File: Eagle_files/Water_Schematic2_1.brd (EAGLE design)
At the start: 25.7 x 32.6 mm, 8 parts

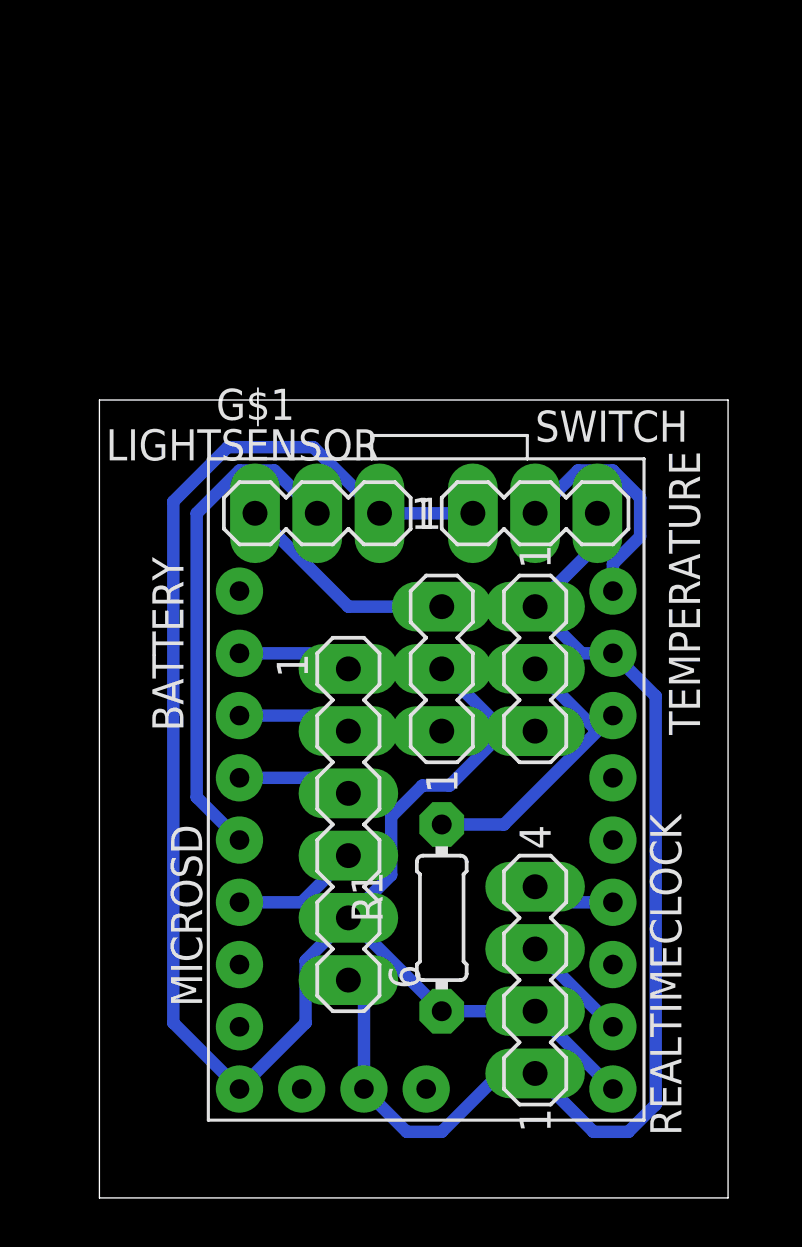
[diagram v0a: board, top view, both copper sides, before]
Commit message: Eagle files updated
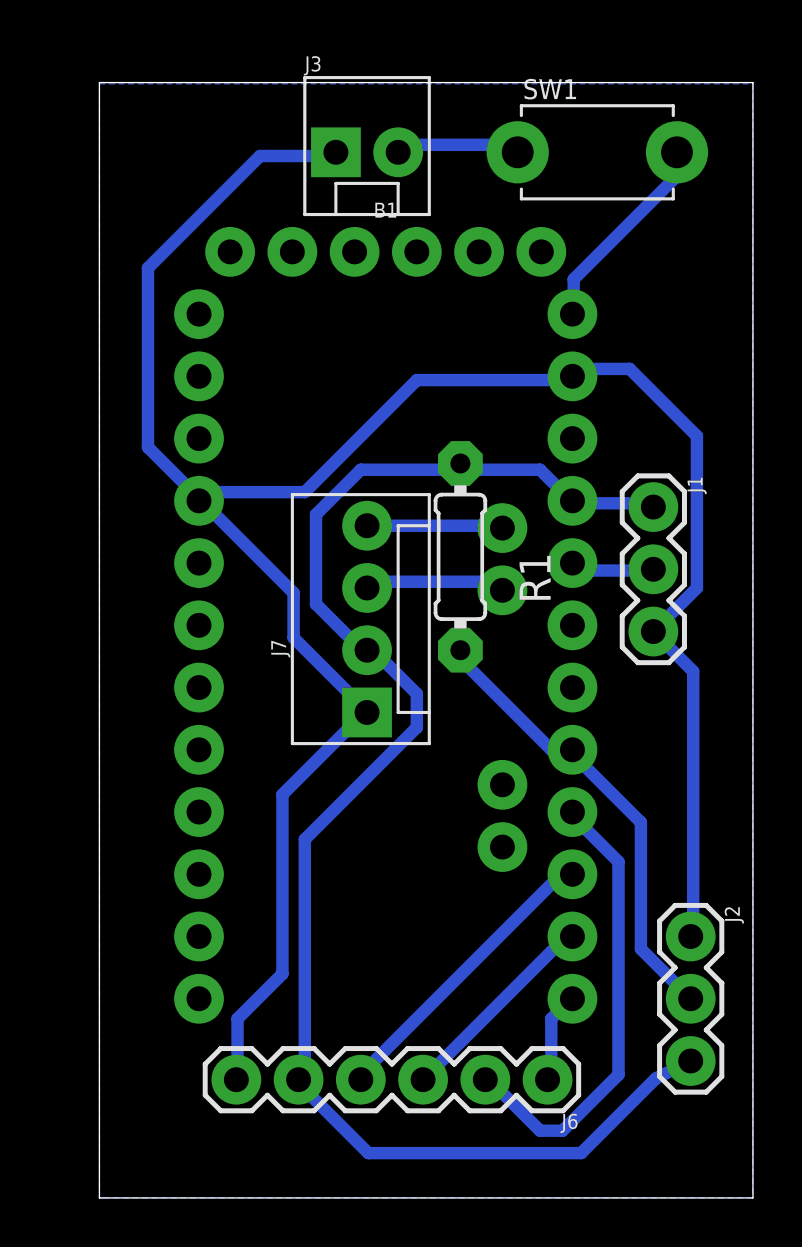
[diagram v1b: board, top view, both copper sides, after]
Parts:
- removed BATTERY, LIGHTSENSOR, SWITCH, TEMPERATURE: (no value), con-lstb:MA03-1
- removed MICROSD: (no value), con-lstb:MA06-1
- removed REALTIMECLOCK: (no value), con-lstb:MA04-1
- removed U$1: DIGISPARK_PRO, digistump:DIGISPARK_PRO
- added B1: ARDUINO_PRO_MINI, SparkFun-Boards:ARDUINO_PRO_MINI
- added J1: Light, SparkFun-Connectors:1X03
- added J2: Temp, SparkFun-Connectors:1X03
- added J3: Battery, SparkFun-Connectors:MOLEX-1X2
- added J6: SD, SparkFun-Connectors:1X06
- added J7: RTC, SparkFun-Connectors:MOLEX-1X4
- added SW1: (no value), adafruit:TACT_PANA-EVQ
- moved R1 14.8 mm to (14.7, 26.2), turned to 90 degrees
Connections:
- removed net DATA: LIGHTSENSOR.2, U$1.PA3
- removed net TEMP: R1.1, TEMPERATURE.2, U$1.PA7
- new net A0: B1.17, J2.2, R1.1
- new net A3: B1.20, J1.2
- new net BAT: J3.2, SW1.P$1
- net GND: now also B1.23, B1.4, J1.3, J2.1, J3.1, J6.6, J7.1; no longer BATTERY.3, LIGHTSENSOR.3, MICROSD.6, REALTIMECLOCK.1, SWITCH.3, TEMPERATURE.1, U$1.GND1, U$1.GND2
- net MISO: now also B1.15, J6.4; no longer MICROSD.4, U$1.PA2
- net MOSI: now also B1.14, J6.3; no longer MICROSD.3, U$1.PA4
- net SC: now also B1.13, J6.1; no longer MICROSD.1, U$1.PA6
- net SCK: now also B1.16, J6.2; no longer MICROSD.2, U$1.PA5
- net SCL: now also B1.A5, J7.4; no longer REALTIMECLOCK.4, U$1.PB2
- net SDA: now also B1.A4, J7.3; no longer REALTIMECLOCK.3, U$1.PB0
- net VCC: now also B1.21, J1.1, J2.3, J6.5, J7.2; no longer BATTERY.2, LIGHTSENSOR.1, MICROSD.5, REALTIMECLOCK.2, SWITCH.1, TEMPERATURE.3, U$1.VCC1, U$1.VCC3
- net VIN: now also B1.24, SW1.P$2; no longer SWITCH.2, U$1.VIN1
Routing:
- net GND: track 60.9 -> 94.9 mm
- net DATA: track 20.4 -> 0.00 mm
- net A0: track 0.00 -> 18.6 mm
- net VCC: track 77.6 -> 61.2 mm
- net SCK: track 4.71 -> 18.7 mm
- net TEMP: track 13.1 -> 0.00 mm
- net MISO: track 5.23 -> 12.3 mm
- net BAT: track 0.00 -> 5.31 mm
- net MOSI: track 4.71 -> 8.48 mm
- net A3: track 0.00 -> 3.57 mm
- net SCL: track 3.44 -> 5.54 mm
- net VIN: track 9.74 -> 8.36 mm
- net SDA: track 4.49 -> 5.81 mm
- net SC: track 4.71 -> 3.73 mm
- added copper zone on layer 16, net GND
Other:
- board size 25.7 x 32.6 mm -> 26.7 x 45.5 mm
